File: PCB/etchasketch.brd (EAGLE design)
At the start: 160 x 100 mm, 7 parts

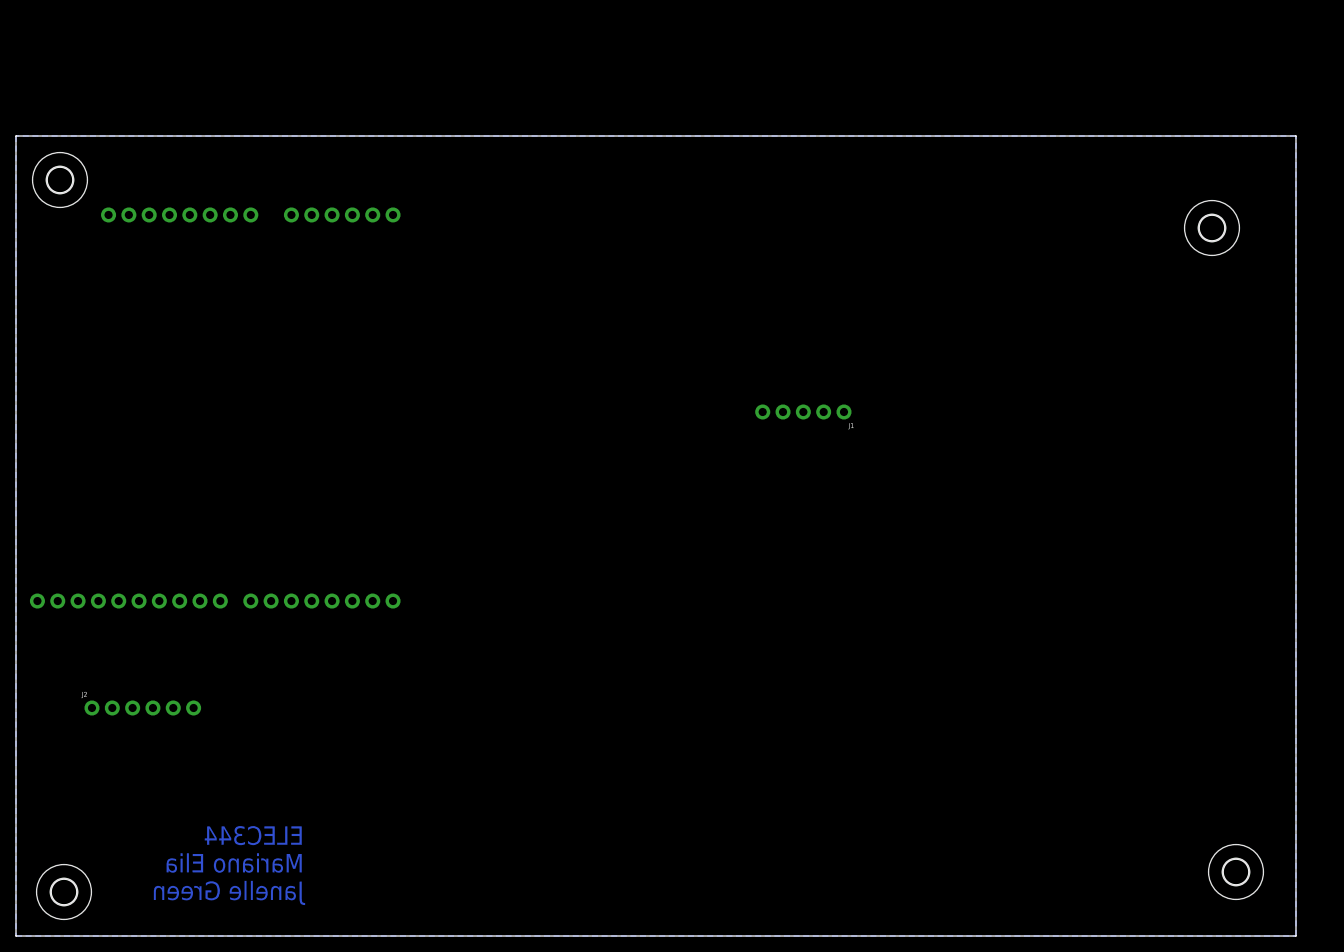
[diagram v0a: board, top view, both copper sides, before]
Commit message: PCB etched
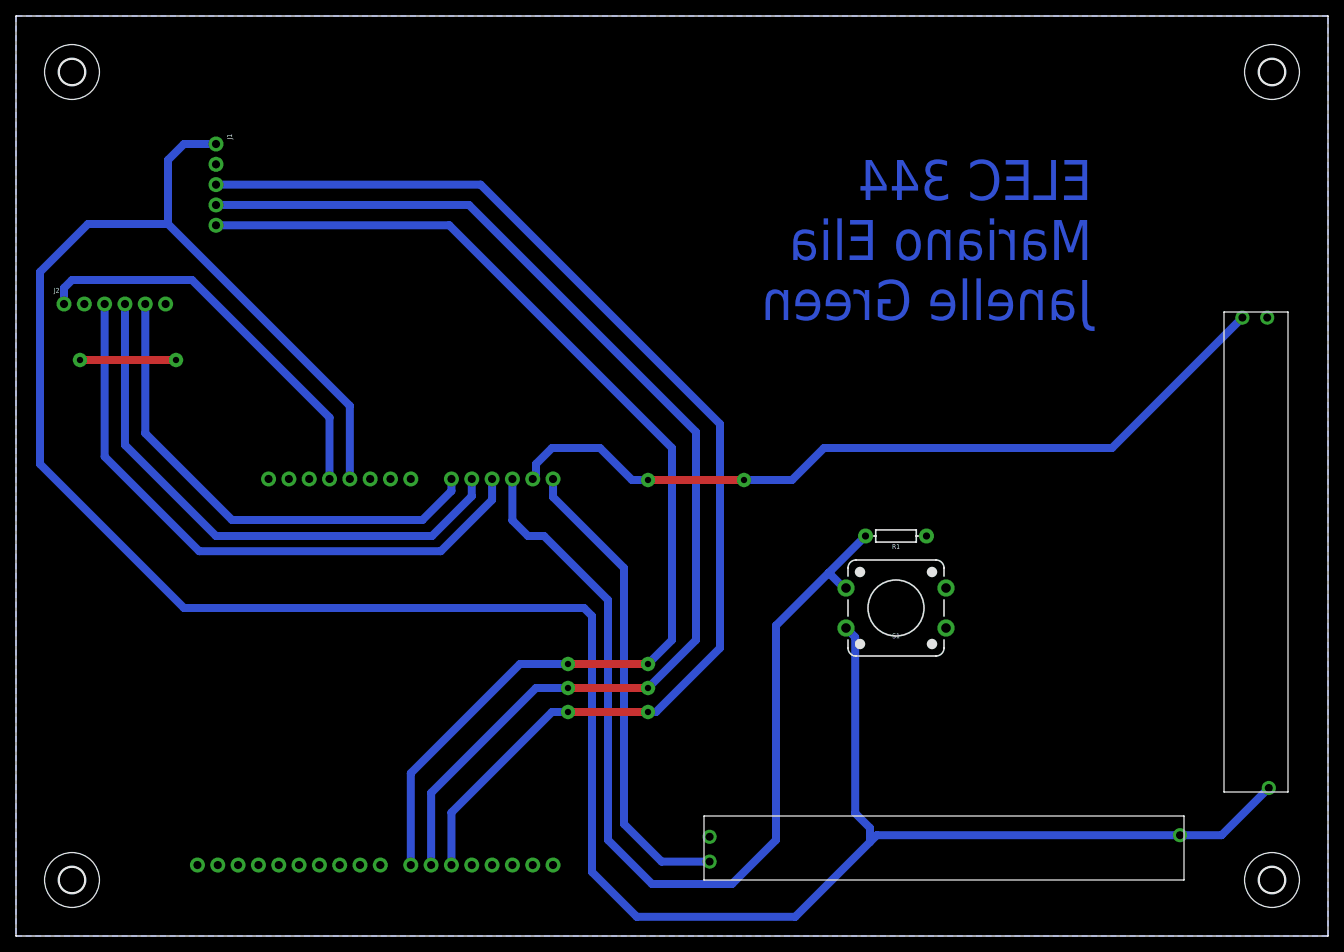
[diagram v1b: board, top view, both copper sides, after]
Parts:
- added R1: 10k, SparkFun-Resistors:AXIAL-0.3
- added S1: MOMENTARY-SWITCH-SPST-PTH-12MM, SparkFun-Switches:TACTILE_SWITCH_PTH_12MM
- added U$1, U$2: 6CMSLIDINGPOT, TPS564208:SLIDINGPOT
- moved J1 85.3 mm to (25.0, 99.0), turned to 270 degrees
- moved J2 50.6 mm to (6.00, 79.0)
- moved B1 38.6 mm to (43.0, 33.0)
- moved H3 20.9 mm to (157.0, 108.0)
- moved H2 13.6 mm to (7.00, 108.0)
- moved H4 4.61 mm to (157.0, 7.00)
- moved H1 1.80 mm to (7.00, 7.00)
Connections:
- new net N$1: B1.A4, U$1.P$2
- new net N$2: B1.A3, R1.P$2, S1.1
- new net N$6: B1.A5, U$2.P$2
- net 5V: now also S1.3, U$1.P$3, U$2.P$3
- net CLK: now also B1.D7
- net CS: now also B1.D6
- net DIN: now also B1.D5
- net GND: now also R1.P$1, U$1.P$1, U$2.P$1
- net XDIR: now also B1.A2
- net YDIR: now also B1.A1
- net ZDIR: now also B1.A0
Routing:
- net 5V: track 0.00 -> 329.1 mm
- net DIN: track 0.00 -> 152.0 mm, vias 0 -> 2
- net CS: track 0.00 -> 147.8 mm, vias 0 -> 2
- net CLK: track 0.00 -> 143.6 mm, vias 0 -> 2
- net N$2: track 0.00 -> 122.4 mm
- net N$1: track 0.00 -> 101.2 mm, vias 0 -> 2
- net XDIR: track 0.00 -> 77.7 mm
- net YDIR: track 0.00 -> 69.9 mm
- net ZDIR: track 0.00 -> 61.9 mm
- net N$6: track 0.00 -> 59.5 mm
- net 3.3V: track 0.00 -> 50.4 mm
- net GND: track 0.00 -> 12.0 mm, vias 0 -> 2
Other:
- board size 160 x 100 mm -> 164 x 115 mm
- board text added: "ELEC 344 Mariano Elia Janelle Green"
- board text removed: "ELEC344 Mariano Elia Janelle Green"
